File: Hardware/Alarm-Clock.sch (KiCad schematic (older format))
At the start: 26 parts, among them IC1 MEGA8-AI, Q1 16Mhz, X1 MINI-USB-32005-201

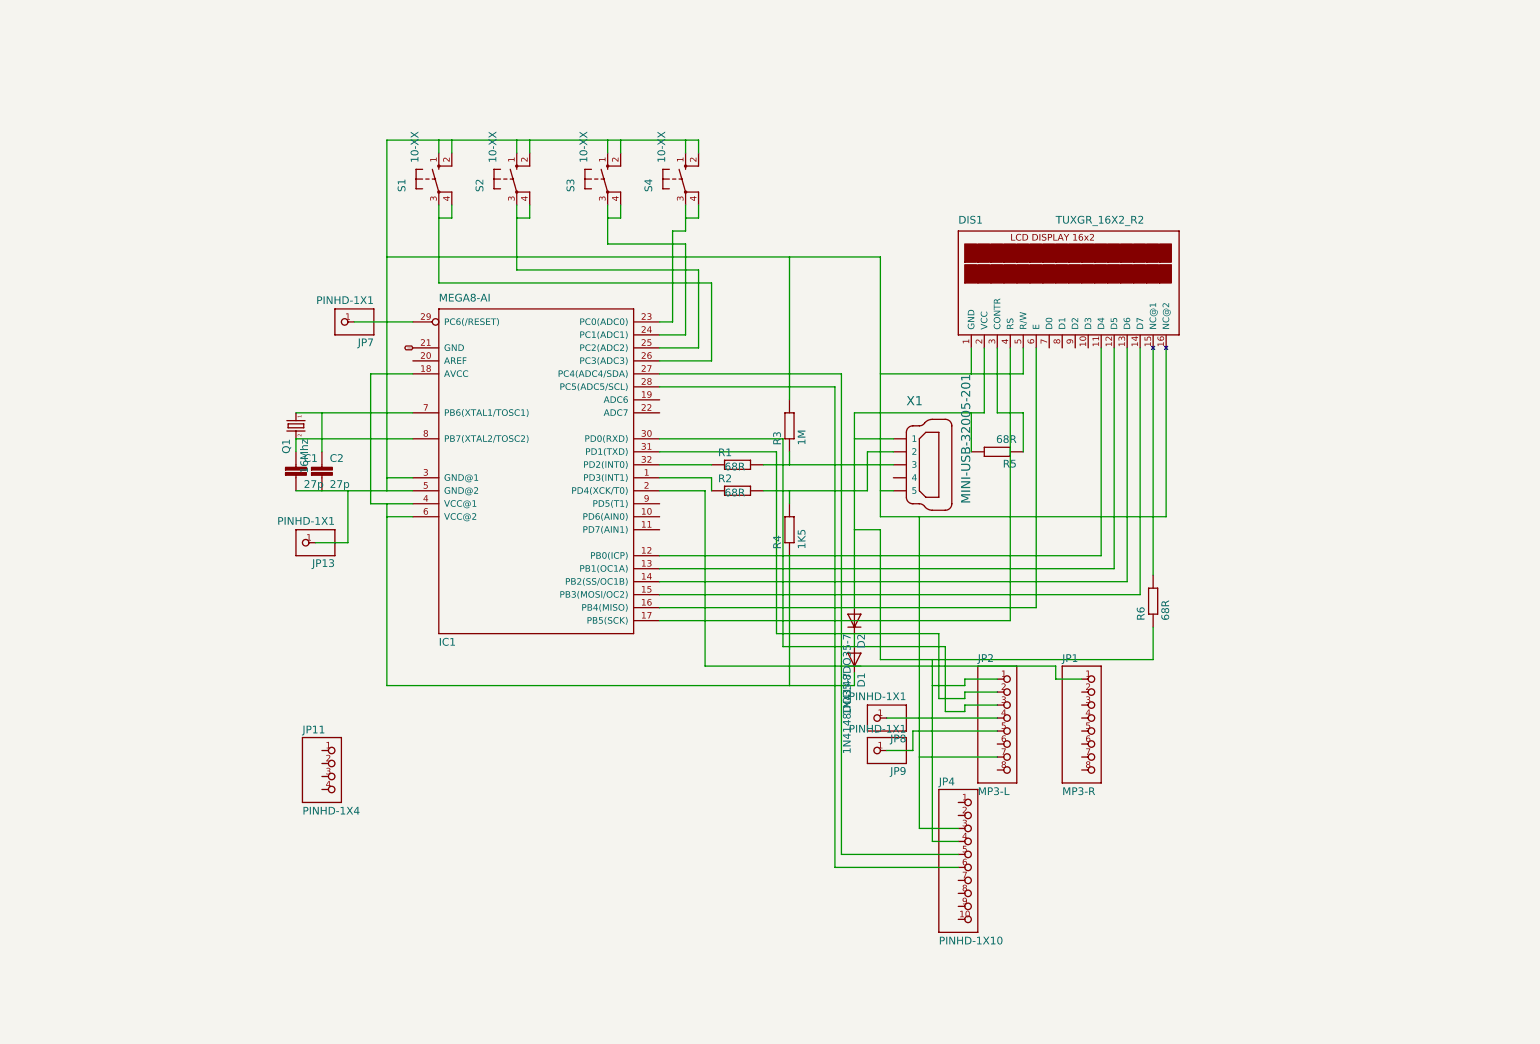
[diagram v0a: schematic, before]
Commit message: update schematic and board
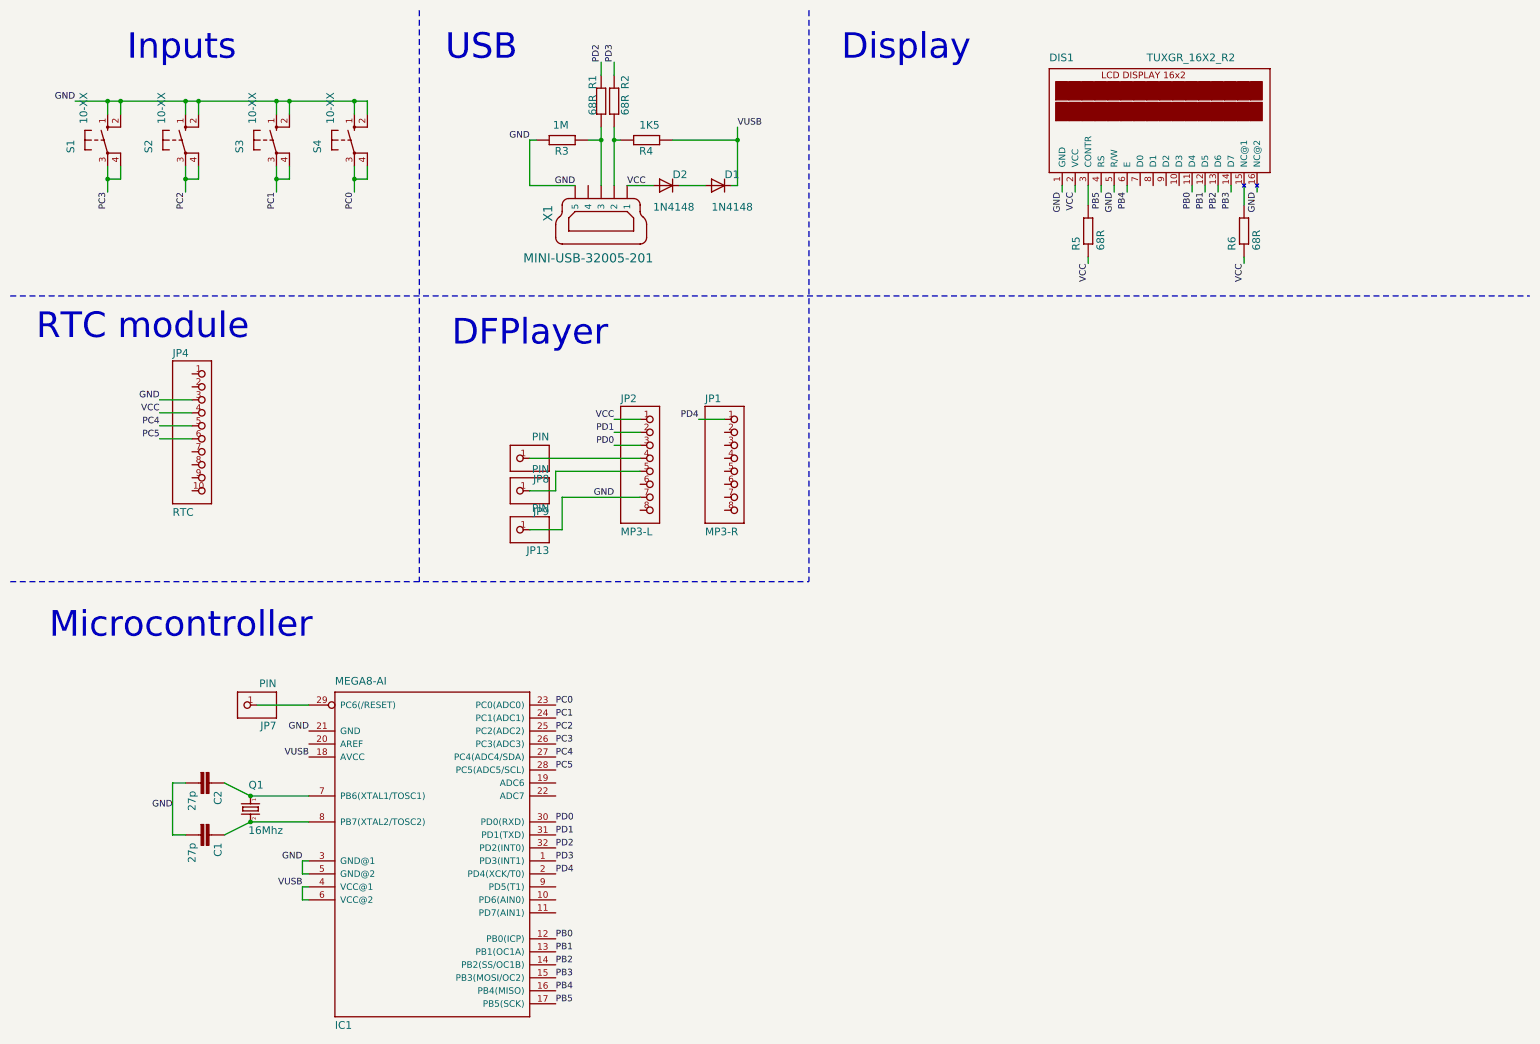
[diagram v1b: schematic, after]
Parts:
- removed JP11: PINHD-1X4, Alarm-Clock:1X04, symbol Alarm-Clock-eagle-import:PINHD-1X4
- D1, D2: value 1N4148DO35-7 -> 1N4148
- JP13, JP7, JP8, JP9: value PINHD-1X1 -> PIN
- JP4: value PINHD-1X10 -> RTC
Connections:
- net GND: now also C1.2, C2.2, DIS1.1 (GND), DIS1.16 (NC@2), DIS1.5 (R/W), IC1.3 (GND@1), IC1.5 (GND@2), JP13.1, JP2.7, JP4.3, R3.2, S1.1 (S), S1.2 (S1), S2.1 (S), S2.2 (S1), S3.1 (S), S3.2 (S1), S4.1 (S), S4.2 (S1), X1.5
- net VCC: now reaches D2.A, DIS1.2 (VCC), JP2.1, JP4.4, R6.1, X1.1
- net VCC: now also R5.1; no longer R5.2
- net PC4: now reaches IC1.27 (PC4(ADC4/SDA)), JP4.5
- net PC5: now reaches IC1.28 (PC5(ADC5/SCL)), JP4.6
- net PD3: now reaches IC1.1 (PD3(INT1)), R2.1
- net PB0: now reaches DIS1.11 (D4), IC1.12 (PB0(ICP))
- net PB1: now reaches DIS1.12 (D5), IC1.13 (PB1(OC1A))
- net PB2: now reaches DIS1.13 (D6), IC1.14 (PB2(SS/OC1B))
- net PB3: now reaches DIS1.14 (D7), IC1.15 (PB3(MOSI/OC2))
- net PB4: now reaches DIS1.6 (E), IC1.16 (PB4(MISO))
- net PB5: now reaches DIS1.4 (RS), IC1.17 (PB5(SCK))
- net VUSB: now reaches D1.C, IC1.18 (AVCC), IC1.4 (VCC@1), IC1.6 (VCC@2), R4.1
- net PD4: now reaches IC1.2 (PD4(XCK/T0)), JP1.1
- net PC0: now reaches IC1.23 (PC0(ADC0)), S4.3 (P), S4.4 (P1)
- net PC1: now reaches IC1.24 (PC1(ADC1)), S3.3 (P), S3.4 (P1)
- net PC2: now reaches IC1.25 (PC2(ADC2)), S2.3 (P), S2.4 (P1)
- net PC3: now reaches IC1.26 (PC3(ADC3)), S1.3 (P), S1.4 (P1)
- net PD0: now reaches IC1.30 (PD0(RXD)), JP2.3
- net PD1: now reaches IC1.31 (PD1(TXD)), JP2.2
- net PD2: now reaches IC1.32 (PD2(INT0)), R1.1
- net at DIS1.3 (CONTR): now also R5.2; no longer R5.1
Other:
- note added: "DFPlayer"
- note added: "Display"
- note added: "Inputs"
- note added: "Microcontroller"
- note added: "RTC module"
- note added: "USB"
- moved on the sheet: C1, C2, D1, D2, DIS1, IC1, JP1, JP13, JP2, JP4, JP7, JP8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
